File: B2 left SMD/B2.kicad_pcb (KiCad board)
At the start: 2 copper layers, 82.8 x 34.7 mm, 1 part

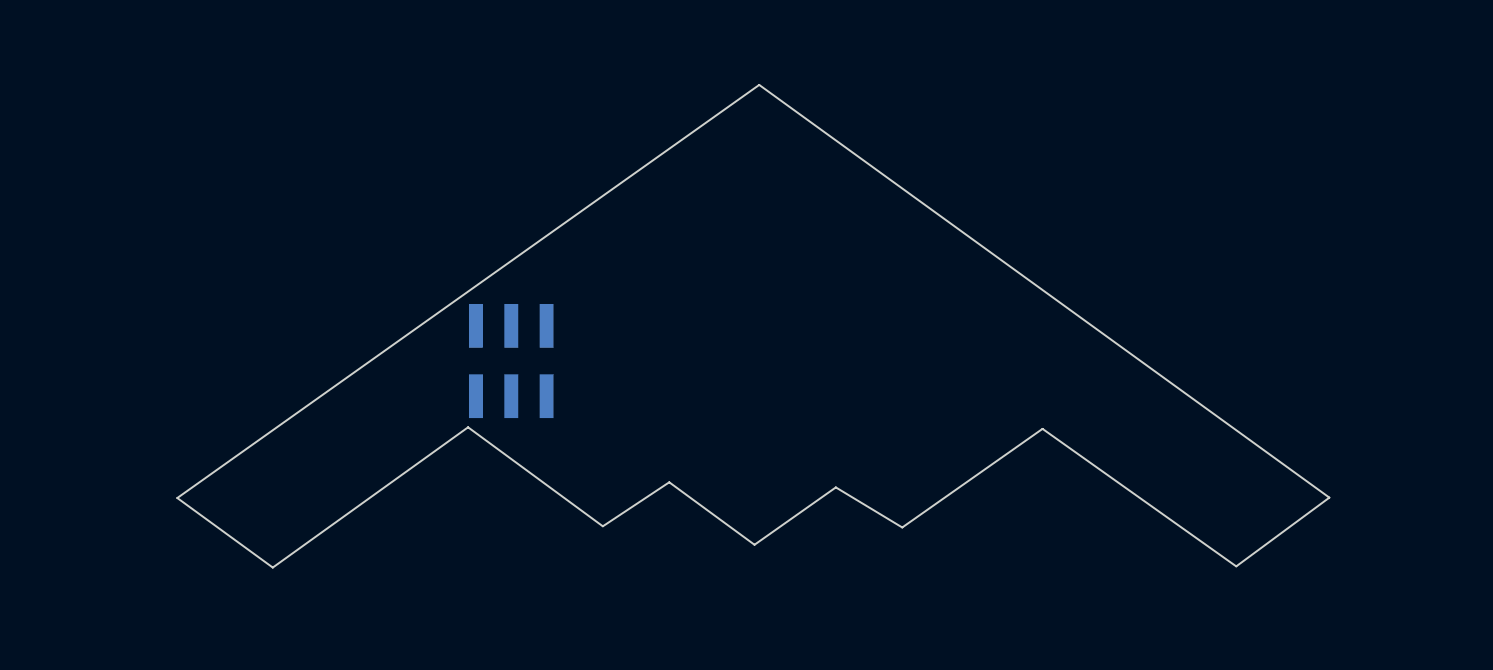
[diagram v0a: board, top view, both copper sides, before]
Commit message: v2 of B2 SAO
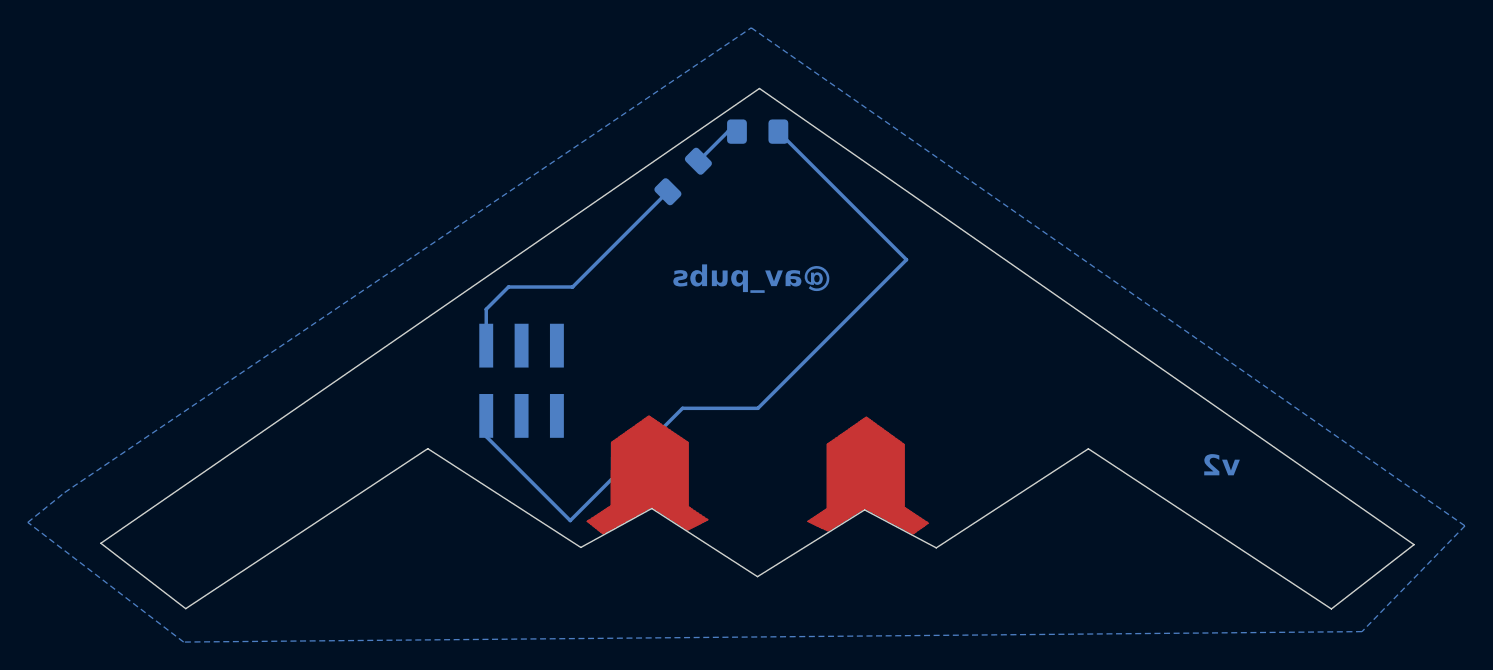
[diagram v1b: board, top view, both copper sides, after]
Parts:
- added REF**: R_1206_3216Metric_Pad1.30x1.75mm_HandSolder, Resistor_SMD:R_1206_3216Metric_Pad1.30x1.75mm_HandSolder, B.Cu at (145.0, 81.9)
- added REF**: LED_1206_3216Metric_Pad1.42x1.75mm_HandSolder, LED_SMD:LED_1206_3216Metric_Pad1.42x1.75mm_HandSolder, B.Cu at (150.3, 78.7)
- moved REF** 1.60 mm to (133.3, 96.6)
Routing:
- net (no net): track 0.00 -> 80.1 mm
- added copper zone on B.Cu, net (none)
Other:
- board size 82.8 x 34.7 mm -> 94.4 x 37.4 mm
- board text added: "v2"
- board text removed: "v1c"
